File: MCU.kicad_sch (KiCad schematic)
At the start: 39 parts, among them J301 SWD, J302 USB4085-GF-A_REVA4, SW301 SW_SPDT, U301 STM32F405RGT6, U302 USBLC6-2SC6, Y301 16MHz

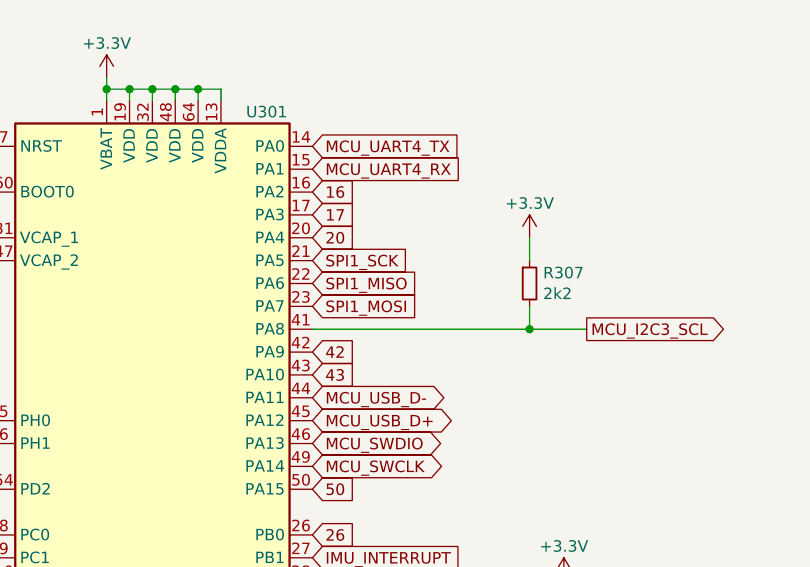
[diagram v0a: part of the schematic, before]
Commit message: sdgnseiogniosegn
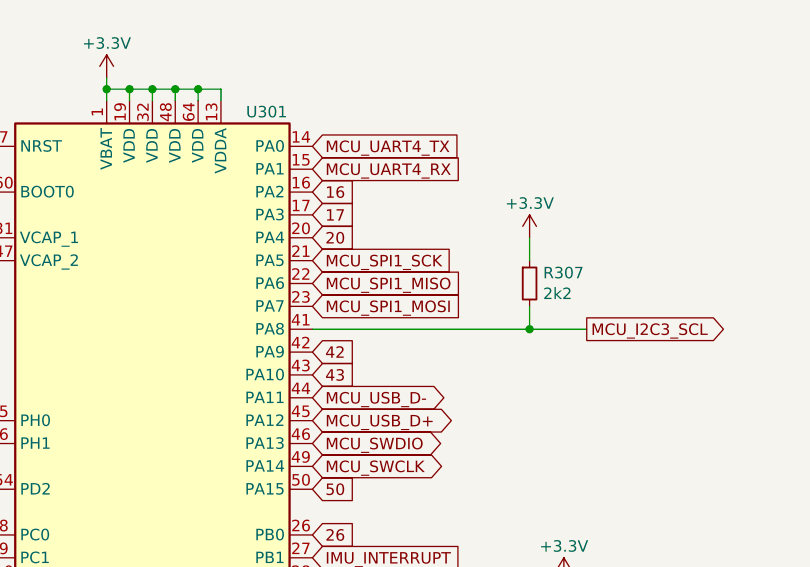
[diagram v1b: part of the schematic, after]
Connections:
- net SPI1_MISO renamed MCU_SPI1_MISO
- net SPI1_MOSI renamed MCU_SPI1_MOSI
- net SPI1_SCK renamed MCU_SPI1_SCK
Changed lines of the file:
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@@
     )
   )
-  (global_label "SPI1_MISO" (shape input) (at 101.6 93.98 0) (fields_autoplaced)
-    (effects (font (size 1.27 1.27)) (justify left))
-    (property "Intersheet References" "${INTERSHEET_REFS}" (id 0) (at 113.7818 94.0594 0)
+  (global_label "MCU_SPI1_MISO" (shape input) (at 101.6 93.98 0) (fields_autoplaced)
+    (effects (font (size 1.27 1.27)) (justify left))
+    (property "Intersheet References" "${INTERSHEET_REFS}" (id 0) (at 118.8013 93.9006 0)
       (effects (font (size 1.27 1.27)) (justify left) hide)
     )
@@
     )
   )
-  (global_label "SPI1_SCK" (shape input) (at 101.6 91.44 0) (fields_autoplaced)
-    (effects (font (size 1.27 1.27)) (justify left))
-    (property "Intersheet References" "${INTERSHEET_REFS}" (id 0) (at 112.9352 91.5194 0)
+  (global_label "MCU_SPI1_SCK" (shape input) (at 101.6 91.44 0) (fields_autoplaced)
+    (effects (font (size 1.27 1.27)) (justify left))
+    (property "Intersheet References" "${INTERSHEET_REFS}" (id 0) (at 117.9547 91.3606 0)
       (effects (font (size 1.27 1.27)) (justify left) hide)
     )
@@
     )
   )
-  (global_label "SPI1_MOSI" (shape input) (at 101.6 96.52 0) (fields_autoplaced)
-    (effects (font (size 1.27 1.27)) (justify left))
-    (property "Intersheet References" "${INTERSHEET_REFS}" (id 0) (at 113.7818 96.5994 0)
-      (effects (font (size 1.27 1.27)) (justify left) hide)
-    )
+  (global_label "MCU_SPI1_MOSI" (shape input) (at 101.6 96.52 0) (fields_autoplaced)
+    (effects (font (size 1.27 1.27)) (justify left))
+    (property "Intersheet References" "${INTERSHEET_REFS}" (id 0) (at 118.8013 96.4406 0)
+      (effects (font (size 1.27 1.27)) (justify left) hide)
+    )
